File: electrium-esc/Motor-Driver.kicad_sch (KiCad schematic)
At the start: 42 parts, among them U2 DRV8301DCAR

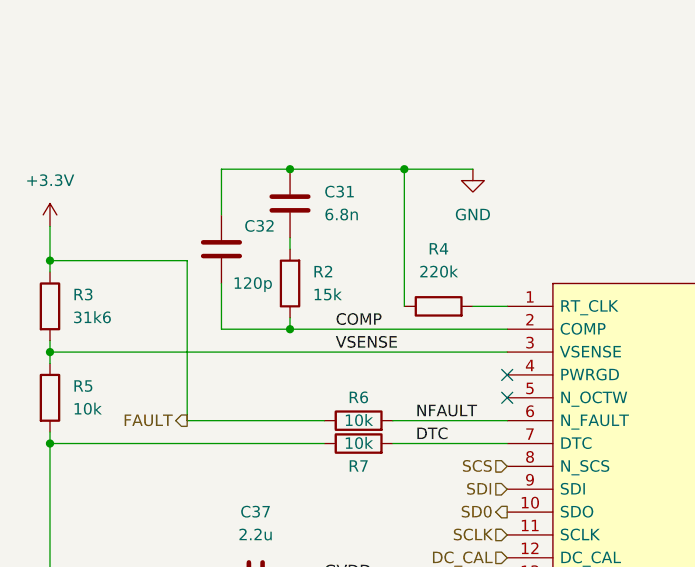
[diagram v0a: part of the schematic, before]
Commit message: Semi-finished schematic
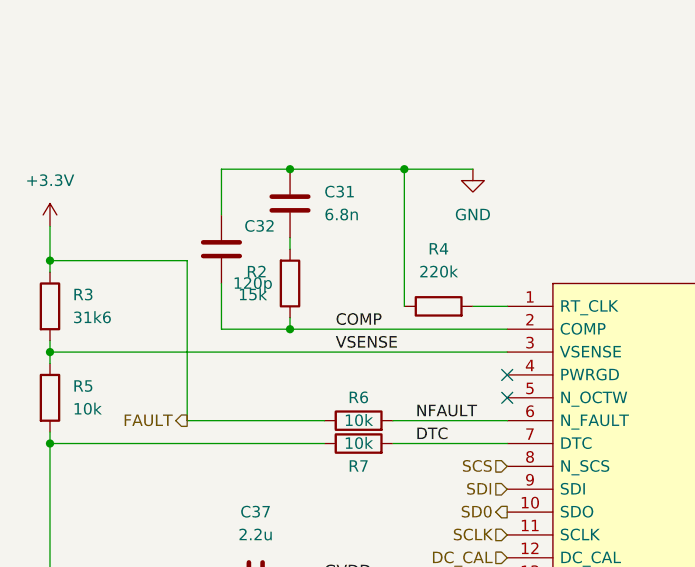
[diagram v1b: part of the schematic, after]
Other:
- moved on the sheet: R2
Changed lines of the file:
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@@
     (pin "2")
   )
-  (symbol (lib_id "Device:R") (at 90.17 67.31 180) (unit 1)
+  (symbol (lib_id "Device:R") (at 90.17 67.31 0) (mirror x) (unit 1)
     (in_bom yes) (on_board yes) (fields_autoplaced)
-    (property "Reference" "R2" (id 0) (at 92.71 66.0399 0)
+    (property "Reference" "R2" (id 0) (at 87.63 66.0399 0)
       (effects (font (size 1.27 1.27)) (justify right))
     )
-    (property "Value" "15k" (id 1) (at 92.71 68.5799 0)
+    (property "Value" "15k" (id 1) (at 87.63 68.5799 0)
       (effects (font (size 1.27 1.27)) (justify right))
     )
-    (property "Footprint" "Resistor_SMD:R_0603_1608Metric" (id 2) (at 91.948 67.31 90)
+    (property "Footprint" "Resistor_SMD:R_0603_1608Metric" (id 2) (at 88.392 67.31 90)
       (effects (font (size 1.27 1.27)) hide)
     )

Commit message: Update more components and few traces
Final design hopefully done by tomorrow. Logistical problems are coming through, needs to suit components to those needs
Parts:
- D1: footprint Diode_THT:D_DO-41_SOD81_P10.16mm_Horizontal -> Diode_SMD:D_0603_1608Metric
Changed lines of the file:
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@@
       (effects (font (size 1.27 1.27)) (justify left))
     )
-    (property "Footprint" "Diode_THT:D_DO-41_SOD81_P10.16mm_Horizontal" (id 2) (at 175.895 86.36 0)
+    (property "Footprint" "Diode_SMD:D_0603_1608Metric" (id 2) (at 175.895 86.36 0)
       (effects (font (size 1.27 1.27)) hide)
     )

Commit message: Add power connections
I realize Vias are unrealistic, need to redo.
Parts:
- D1: footprint Diode_SMD:D_0603_1608Metric -> Diode_SMD:D_SOD-123
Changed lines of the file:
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@@
       (effects (font (size 1.27 1.27)) (justify left))
     )
-    (property "Footprint" "Diode_SMD:D_0603_1608Metric" (id 2) (at 175.895 86.36 0)
+    (property "Footprint" "Diode_SMD:D_SOD-123" (id 2) (at 175.895 86.36 0)
       (effects (font (size 1.27 1.27)) hide)
     )

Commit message: Fix most ERC errors, just some connections now!
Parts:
- L1: footprint Inductor_SMD:L_Vishay_IHLP-2020 -> Inductor_SMD:L_Taiyo-Yuden_NR-30xx
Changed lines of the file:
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@@
     (property "Reference" "L1" (id 0) (at 190.5 77.47 0))
     (property "Value" "22u" (id 1) (at 190.5 81.28 0))
-    (property "Footprint" "Inductor_SMD:L_Vishay_IHLP-2020" (id 2) (at 190.5 80.01 0)
+    (property "Footprint" "Inductor_SMD:L_Taiyo-Yuden_NR-30xx" (id 2) (at 190.5 80.01 0)
       (effects (font (size 1.27 1.27)) hide)
     )

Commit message: Add Gerber and final files
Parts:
- D1: footprint Diode_SMD:D_SOD-123 -> Diode_SMD:D_SMA
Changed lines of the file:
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@@
       (effects (font (size 1.27 1.27)) (justify left))
     )
-    (property "Footprint" "Diode_SMD:D_SOD-123" (id 2) (at 175.895 86.36 0)
+    (property "Footprint" "Diode_SMD:D_SMA" (id 2) (at 175.895 86.36 0)
       (effects (font (size 1.27 1.27)) hide)
     )
